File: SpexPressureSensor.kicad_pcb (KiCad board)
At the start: 2 copper layers, 28 x 28 mm, 28 parts, among them P1 CONN_6, P2 NICHROME, P3 TC2030-CTX, Q1 IRLL3303PbF, U1 ST1480ABDR, U2 TPS769XX, U3 MKL03ZxxVFG4, U4 BME280, U7 LT6105

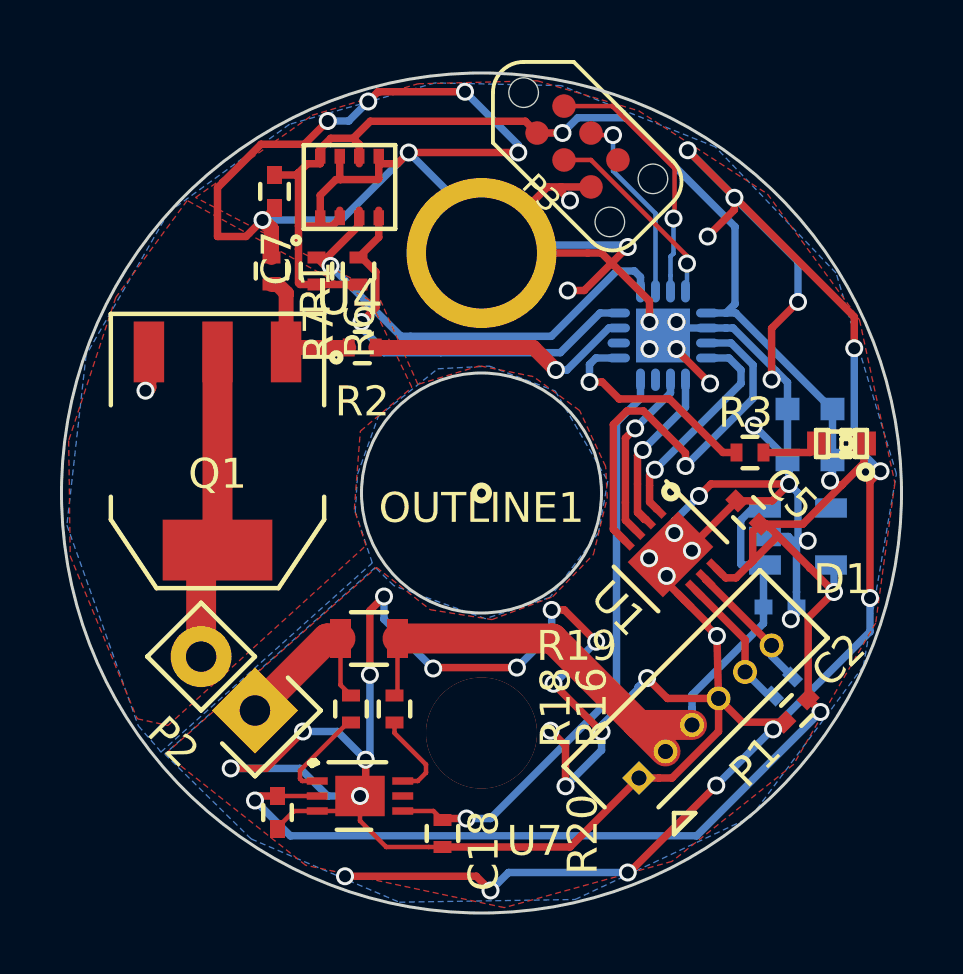
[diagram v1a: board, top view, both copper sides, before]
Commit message: Fixed some issues
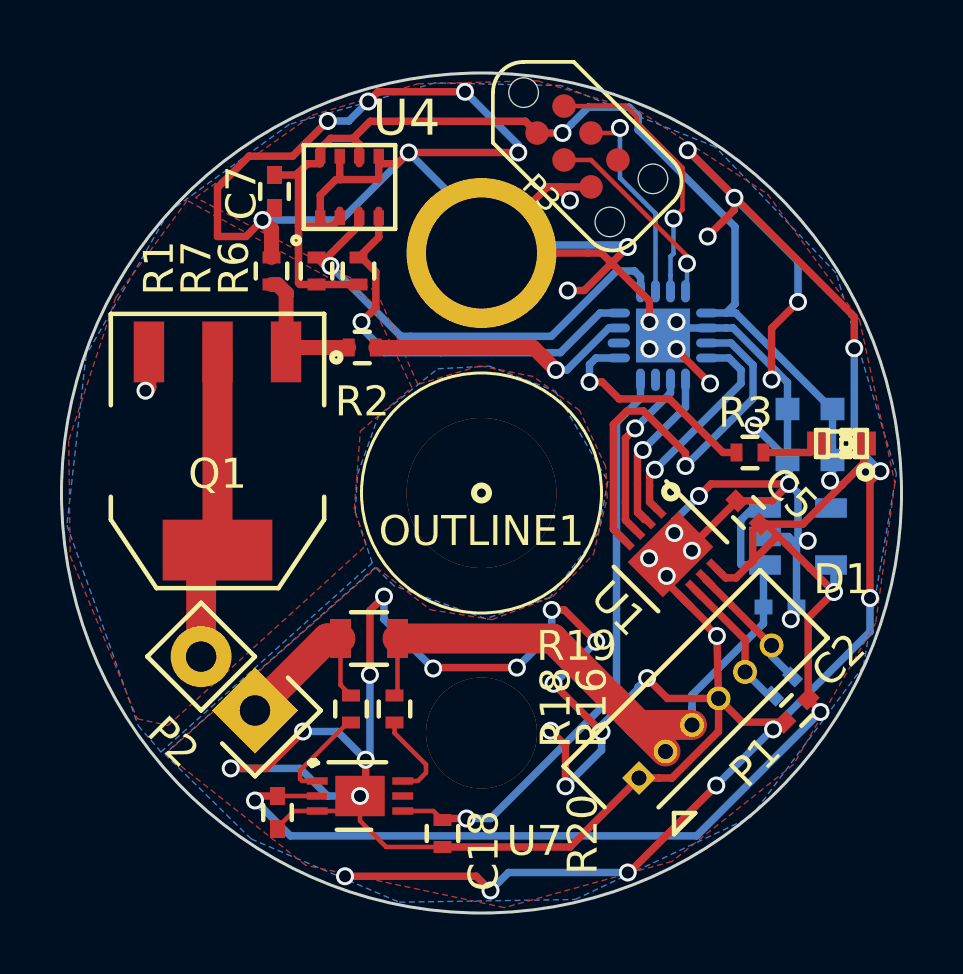
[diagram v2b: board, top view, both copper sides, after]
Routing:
- net +3.3V: track 79.3 -> 79.8 mm
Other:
- outline, holes or cut-outs redrawn
